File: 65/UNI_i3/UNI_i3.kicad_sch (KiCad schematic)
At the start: 164 parts, among them J1 Conn_01x19_Pin, J2 Conn_01x19_Pin, SW1 MX_SW_solder, SW10 MX_SW_solder, SW11 MX_SW_solder, SW12 MX_SW_solder, SW13 MX_SW_solder, SW14 MX_SW_solder, SW15 MX_SW_solder, SW16 MX_SW_solder, SW17 MX_SW_solder, SW18 MX_SW_solder, SW19 MX_SW_solder, SW2 MX_SW_solder, SW20 MX_SW_solder, SW21 MX_SW_solder, SW22 MX_SW_solder, SW23 MX_SW_solder, SW24 MX_SW_solder, SW25 MX_SW_solder, SW26 MX_SW_solder, SW27 MX_SW_solder, SW28 MX_SW_solder, SW29 MX_SW_solder, SW3 MX_SW_solder, SW30 MX_SW_solder, SW31 MX_SW_solder, SW32 RotaryEncoder_Switch, SW33 MX_SW_solder, SW34 MX_SW_solder, SW35 MX_SW_solder, SW36 MX_SW_solder, SW37 MX_SW_solder, SW38 MX_SW_solder, SW39 MX_SW_solder, SW4 MX_SW_solder, SW40 MX_SW_solder, SW41 MX_SW_solder, SW42 MX_SW_solder, SW43 MX_SW_solder, SW44 MX_SW_solder, SW45 MX_SW_solder, SW46 MX_SW_solder, SW47 MX_SW_solder, SW48 RotaryEncoder_Switch, SW49 MX_SW_solder, SW5 MX_SW_solder, SW50 MX_SW_solder, SW51 MX_SW_solder, SW52 MX_SW_solder, SW53 MX_SW_solder, SW54 MX_SW_solder, SW55 MX_SW_solder, SW56 MX_SW_solder, SW57 MX_SW_solder, SW58 MX_SW_solder, SW59 MX_SW_solder, SW6 MX_SW_solder, SW60 MX_SW_solder, SW61 MX_SW_solder, SW62 MX_SW_solder, SW63 MX_SW_solder, SW64 MX_SW_solder, SW65 MX_SW_solder, SW66 MX_SW_solder, SW67 MX_SW_solder, SW68 MX_SW_solder, SW69 MX_SW_solder, SW7 MX_SW_solder, SW70 MX_SW_solder, SW71 MX_SW_solder, SW72 MX_SW_solder, SW73 MX_SW_solder, SW74 MX_SW_solder, SW75 MX_SW_solder, SW76 SW_Push_45deg, SW8 MX_SW_solder, SW9 MX_SW_solder, U1 Bonsai-C4-extended

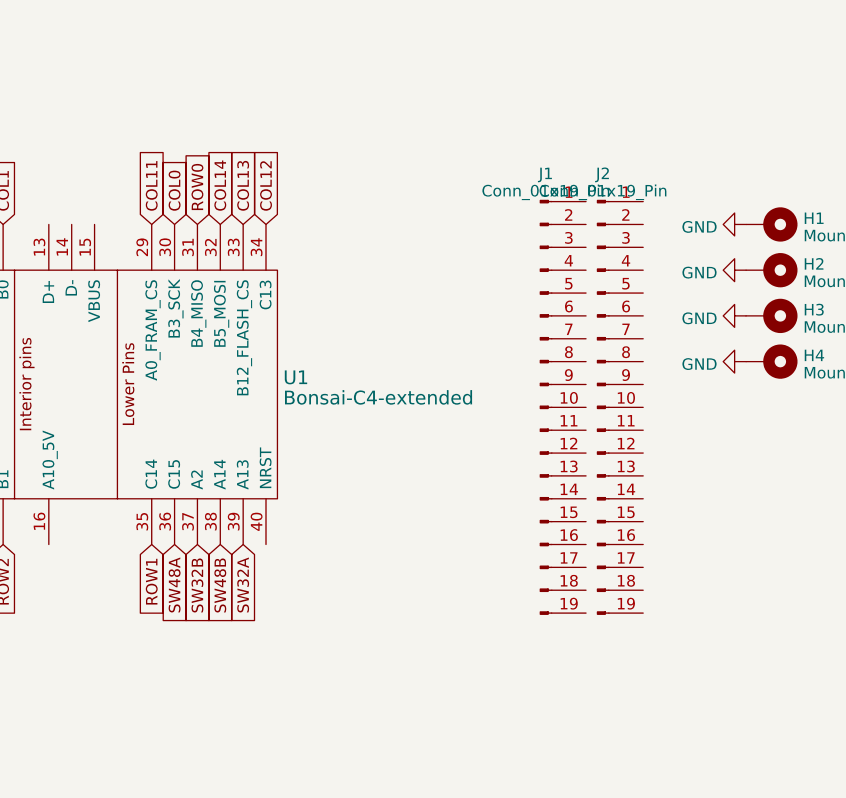
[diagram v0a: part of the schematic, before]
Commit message: working on 60B uni
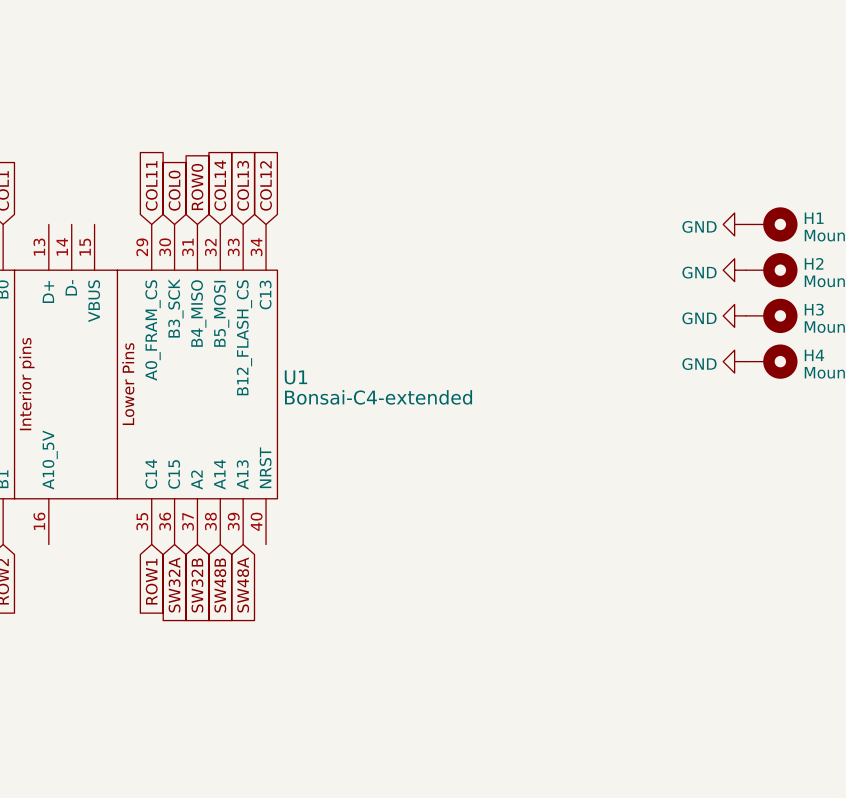
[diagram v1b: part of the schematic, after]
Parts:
- removed J1, J2: Conn_01x19_Pin, Connector_PinHeader_2.54mm:PinHeader_1x19_P2.54mm_Vertical_SMD_Pin1Left, symbol Connector:Conn_01x19_Pin
- U1: footprint shoonies_parts:Bonsai_C4_extended_SMD -> shoonies_parts:Bonsai_C4_extended_THT
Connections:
- net SW32A: now also U1.36 (C15); no longer U1.39 (A13)
- net SW48A: now also U1.39 (A13); no longer U1.36 (C15)
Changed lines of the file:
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@@
     )
   )
-  (global_label "SW32A" (shape input) (at 105.41 213.36 270) (fields_autoplaced)
+  (global_label "SW32A" (shape input) (at 97.79 213.36 270) (fields_autoplaced)
     (effects (font (size 1.27 1.27)) (justify right))
-    (property "Intersheetrefs" "${INTERSHEET_REFS}" (at 105.41 222.4343 90)
-      (effects (font (size 1.27 1.27)) (justify right) hide)
+    (property "Intersheetrefs" "${INTERSHEET_REFS}" (at 97.79 222.4343 90)
+      (effects (font (size 1.27 1.27)) (justify left) hide)
     )
   )
@@
     )
   )
-  (global_label "SW48A" (shape input) (at 97.79 213.36 270) (fields_autoplaced)
+  (global_label "SW48A" (shape input) (at 105.41 213.36 270) (fields_autoplaced)
     (effects (font (size 1.27 1.27)) (justify right))
-    (property "Intersheetrefs" "${INTERSHEET_REFS}" (at 97.79 222.4343 90)
-      (effects (font (size 1.27 1.27)) (justify left) hide)
+    (property "Intersheetrefs" "${INTERSHEET_REFS}" (at 105.41 222.4343 90)
+      (effects (font (size 1.27 1.27)) (justify right) hide)
     )
   )
@@
     )
   )
-  (symbol (lib_id "Connector:Conn_01x19_Pin") (at 138.43 198.12 0) (unit 1)
-    (in_bom yes) (on_board yes) (dnp no) (fields_autoplaced)
-    (property "Reference" "J1" (at 139.065 172.1739 0)
-      (effects (font (size 1.27 1.27)))
-    )
-    (property "Value" "Conn_01x19_Pin" (at 139.065 174.0949 0)
-      (effects (font (size 1.27 1.27)))
-    )
-    (property "Footprint" "Connector_PinHeader_2.54mm:PinHeader_1x19_P2.54mm_Vertical_SMD_Pin1Left" (at 138.43 198.12 0)
-      (effects (font (size 1.27 1.27)) hide)
-    )
-    (property "Datasheet" "~" (at 138.43 198.12 0)
-      (effects (font (size 1.27 1.27)) hide)
-    )
-    (pin "1")
-    (pin "10")
-    (pin "11")
-    (pin "12")
-    (pin "13")
-    (pin "14")
-    (pin "15")
-    (pin "16")
-    (pin "17")
-    (pin "18")
-    (pin "19")
-    (pin "2")
-    (pin "3")
-    (pin "4")
-    (pin "5")
-    (pin "6")
-    (pin "7")
-    (pin "8")
-    (pin "9")
-    (instances
-      (project "UNI_i3"
-        (path "/6059e08a-17a3-445e-9a30-384483938524"
-          (reference "J1") (unit 1)
-        )
-      )
-    )
-  )
   (symbol (lib_id "marbastlib-mx:MX_SW_solder") (at 148.59 91.44 180) (unit 1)
     (in_bom yes) (on_board yes) (dnp no) (fields_autoplaced)
@@
     )
   )
-  (symbol (lib_id "Connector:Conn_01x19_Pin") (at 144.78 198.12 0) (unit 1)
-    (in_bom yes) (on_board yes) (dnp no) (fields_autoplaced)
-    (property "Reference" "J2" (at 145.415 172.1739 0)
-      (effects (font (size 1.27 1.27)))
-    )
-    (property "Value" "Conn_01x19_Pin" (at 145.415 174.0949 0)
-      (effects (font (size 1.27 1.27)))
-    )
-    (property "Footprint" "Connector_PinHeader_2.54mm:PinHeader_1x19_P2.54mm_Vertical_SMD_Pin1Left" (at 144.78 198.12 0)
-      (effects (font (size 1.27 1.27)) hide)
-    )
-    (property "Datasheet" "~" (at 144.78 198.12 0)
-      (effects (font (size 1.27 1.27)) hide)
-    )
-    (pin "1")
-    (pin "10")
-    (pin "11")
-    (pin "12")
-    (pin "13")
-    (pin "14")
-    (pin "15")
-    (pin "16")
-    (pin "17")
-    (pin "18")
-    (pin "19")
-    (pin "2")
-    (pin "3")
-    (pin "4")
-    (pin "5")
-    (pin "6")
-    (pin "7")
-    (pin "8")
-    (pin "9")
-    (instances
-      (project "UNI_i3"
-        (path "/6059e08a-17a3-445e-9a30-384483938524"
-          (reference "J2") (unit 1)
-        )
-      )
-    )
-  )
   (symbol (lib_id "marbastlib-mx:MX_SW_solder") (at 243.84 53.34 180) (unit 1)
     (in_bom yes) (on_board yes) (dnp no)
@@
       (effects (font (size 1.524 1.524)) (justify right))
     )
-    (property "Footprint" "shoonies_parts:Bonsai_C4_extended_SMD" (at 114.3 195.58 0)
+    (property "Footprint" "shoonies_parts:Bonsai_C4_extended_THT" (at 114.3 195.58 0)
       (effects (font (size 1.524 1.524)) hide)
     )

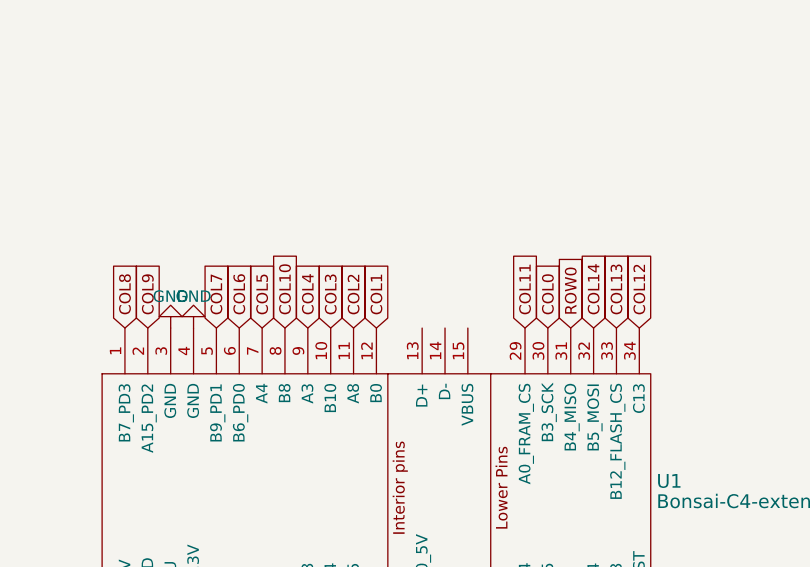
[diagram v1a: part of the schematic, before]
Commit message: UNI/TAKO i3 for production
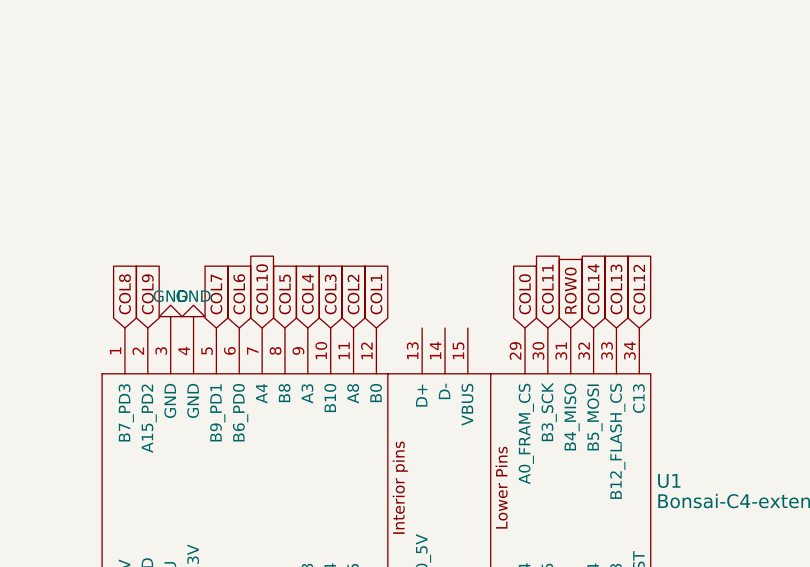
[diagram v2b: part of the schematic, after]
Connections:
- net COL0: now also U1.29 (A0_FRAM_CS); no longer U1.30 (B3_SCK)
- net COL10: now also U1.7 (A4); no longer U1.8 (B8)
- net COL11: now also U1.30 (B3_SCK); no longer U1.29 (A0_FRAM_CS)
- net COL5: now also U1.8 (B8); no longer U1.7 (A4)
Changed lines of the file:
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@@
     )
   )
-  (global_label "COL11" (shape input) (at 95.25 177.8 90) (fields_autoplaced)
+  (global_label "COL11" (shape input) (at 97.79 177.8 90) (fields_autoplaced)
     (effects (font (size 1.27 1.27)) (justify left))
-    (property "Intersheetrefs" "${INTERSHEET_REFS}" (at 95.25 168.8466 90)
-      (effects (font (size 1.27 1.27)) (justify left) hide)
+    (property "Intersheetrefs" "${INTERSHEET_REFS}" (at 97.79 168.8466 90)
+      (effects (font (size 1.27 1.27)) (justify right) hide)
     )
   )
@@
     )
   )
-  (global_label "COL0" (shape input) (at 97.79 177.8 90) (fields_autoplaced)
+  (global_label "COL0" (shape input) (at 95.25 177.8 90) (fields_autoplaced)
     (effects (font (size 1.27 1.27)) (justify left))
-    (property "Intersheetrefs" "${INTERSHEET_REFS}" (at 97.79 170.0561 90)
-      (effects (font (size 1.27 1.27)) (justify left) hide)
+    (property "Intersheetrefs" "${INTERSHEET_REFS}" (at 95.25 170.0561 90)
+      (effects (font (size 1.27 1.27)) (justify right) hide)
     )
   )
@@
     )
   )
-  (global_label "COL10" (shape input) (at 68.58 177.8 90) (fields_autoplaced)
+  (global_label "COL10" (shape input) (at 66.04 177.8 90) (fields_autoplaced)
     (effects (font (size 1.27 1.27)) (justify left))
-    (property "Intersheetrefs" "${INTERSHEET_REFS}" (at 68.58 168.8466 90)
-      (effects (font (size 1.27 1.27)) (justify left) hide)
+    (property "Intersheetrefs" "${INTERSHEET_REFS}" (at 66.04 168.8466 90)
+      (effects (font (size 1.27 1.27)) (justify right) hide)
     )
   )
@@
     )
   )
-  (global_label "COL5" (shape input) (at 66.04 177.8 90) (fields_autoplaced)
+  (global_label "COL5" (shape input) (at 68.58 177.8 90) (fields_autoplaced)
     (effects (font (size 1.27 1.27)) (justify left))
-    (property "Intersheetrefs" "${INTERSHEET_REFS}" (at 66.04 170.0561 90)
-      (effects (font (size 1.27 1.27)) (justify right) hide)
+    (property "Intersheetrefs" "${INTERSHEET_REFS}" (at 68.58 170.0561 90)
+      (effects (font (size 1.27 1.27)) (justify left) hide)
     )
   )
